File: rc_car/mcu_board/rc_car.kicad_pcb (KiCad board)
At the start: 2 copper layers, 31.1 x 36.2 mm, 22 parts, among them J1 Atmega328, P4 CONN_01X03

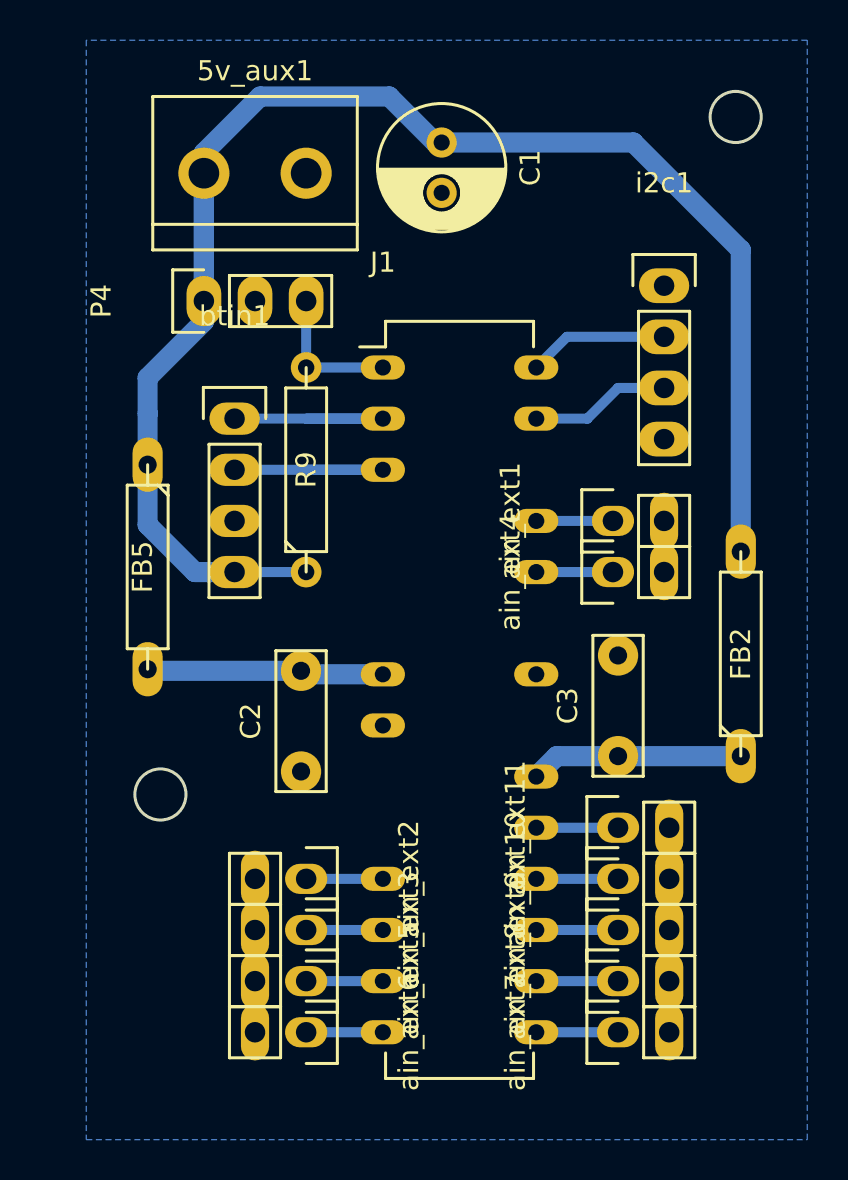
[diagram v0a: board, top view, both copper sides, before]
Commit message: fixes
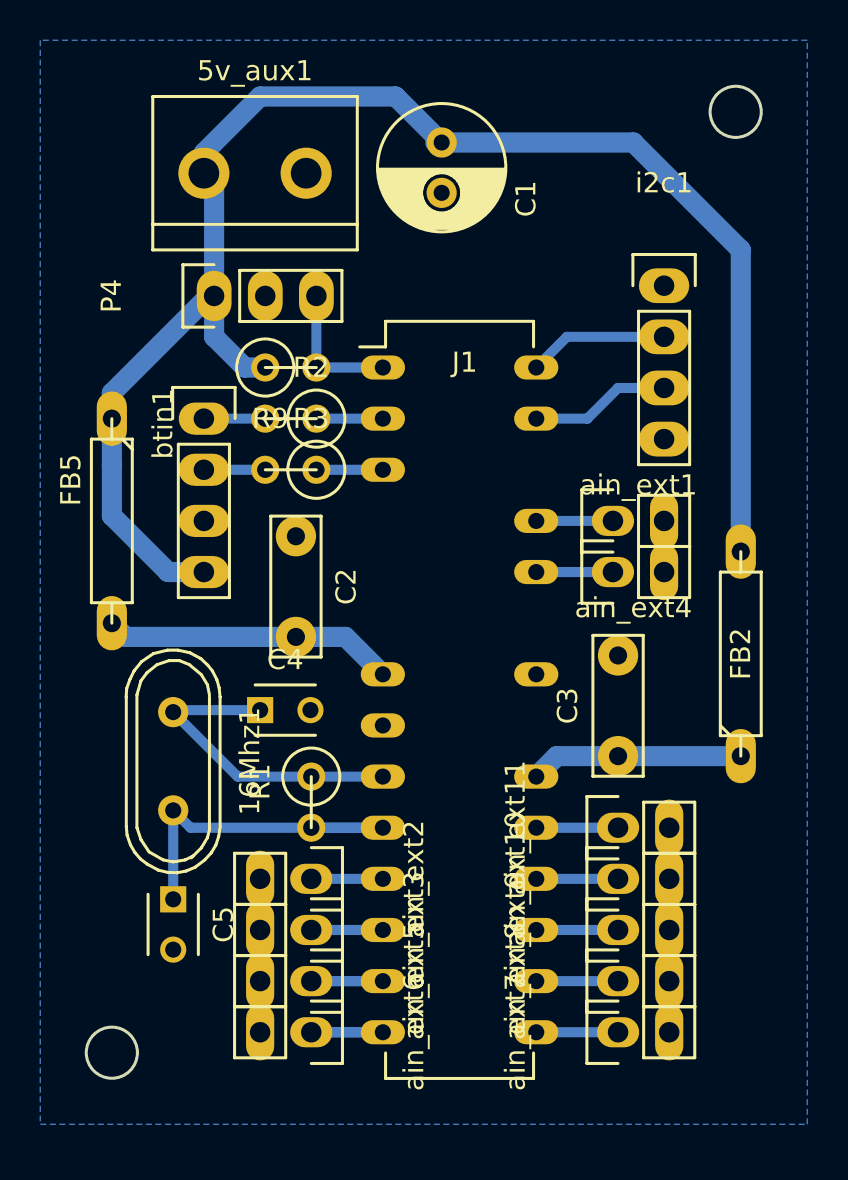
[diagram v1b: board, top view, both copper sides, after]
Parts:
- added 16Mhz1: Crystal_Small, Crystals:Crystal_HC49-U_Vertical, F.Cu at (70.5, 75.8)
- added C4: 22pF, Capacitors_ThroughHole:C_Disc_D3_P2.5, F.Cu at (74.8, 73.3)
- added C5: 22pF, Capacitors_ThroughHole:C_Disc_D3_P2.5, F.Cu at (70.5, 82.7)
- added R1: 1M, Discret:R1, F.Cu at (77.3, 77.9)
- added R2: 1K, Discret:R1, F.Cu at (76.3, 58.8)
- added R3: 1K, Discret:R1, F.Cu at (76.3, 61.3)
- R9: footprint Discret:R4 -> Discret:R1
- moved C2 11.7 mm to (76.6, 64.6), turned to 270 degrees
- moved R9 5.14 mm to (76.3, 56.3), turned to 0 degrees
- moved FB5 2.90 mm to (67.4, 63.9)
- moved btin1 1.52 mm to (72.0, 58.8)
- moved P4 0.57 mm to (72.5, 52.7)
- moved ain_ext2 0.25 mm to (77.3, 81.7)
- moved ain_ext3 0.25 mm to (77.3, 84.2)
- moved ain_ext5 0.25 mm to (77.3, 86.7)
- moved ain_ext6 0.25 mm to (77.3, 89.3)
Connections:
- J1 pad 2: /RX -> Net-(J1-Pad2)
- J1 pad 3: /TX -> Net-(J1-Pad3)
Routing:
- net Net-(16Mhz1-Pad2): track 0.00 -> 18.3 mm
- net Net-(16Mhz1-Pad1): track 0.00 -> 16.1 mm
- net /TX: track 11.2 -> 3.05 mm
- net /RX: track 11.2 -> 3.05 mm
- net /D4: track 3.94 -> 7.49 mm
- net /D3: track 3.81 -> 7.37 mm
- net /D2: track 3.81 -> 7.37 mm
- net Net-(J1-Pad3): track 0.00 -> 3.30 mm
- net Net-(J1-Pad2): track 0.00 -> 3.30 mm
- net /5V: track 83.0 -> 80.5 mm
- net Net-(C2-Pad2): track 12.0 -> 14.5 mm
- net /RST: track 7.58 -> 6.86 mm
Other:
- board size 31.1 x 36.2 mm -> 33.5 x 49.3 mm

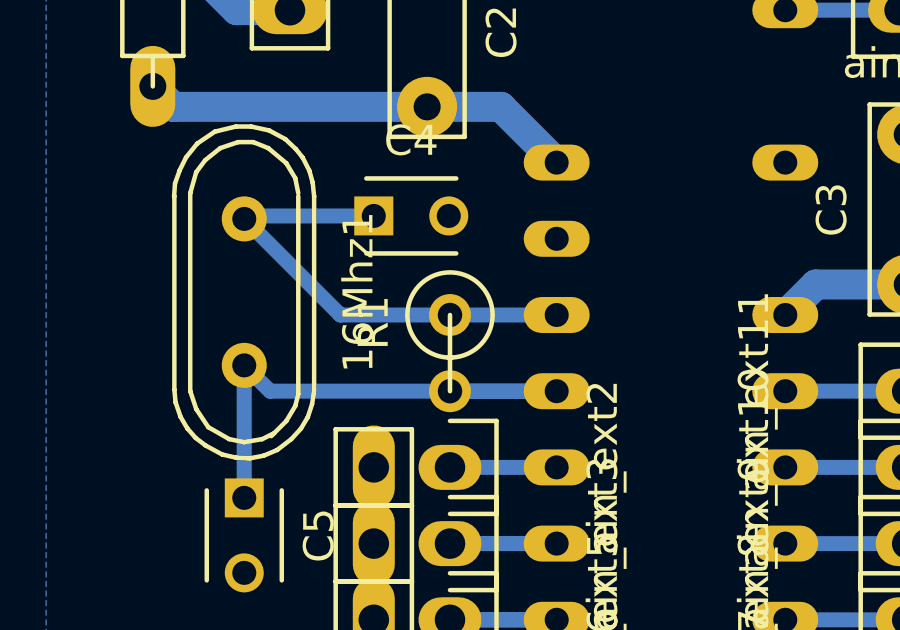
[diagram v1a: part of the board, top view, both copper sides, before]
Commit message: updates
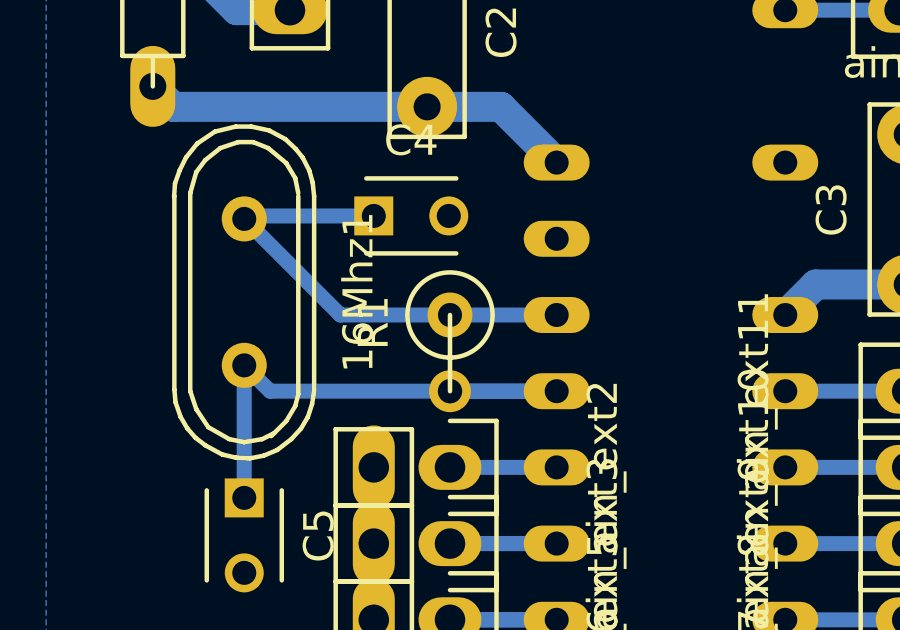
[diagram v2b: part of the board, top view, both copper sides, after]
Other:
- rule pad_to_mask_clearance: 0.2 -> 0
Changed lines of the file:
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@@
-(kicad_pcb (version 4) (host pcbnew 4.0.6)
+(kicad_pcb (version 20171130) (host pcbnew 5.1.4-e60b266~84~ubuntu18.04.1)
   (general
-    (links 57)
-    (no_connects 0)
-    (area 62.36 39.754 101.981001 93.853001)
-    (thickness 1.6)
+    (thickness 1)
     (drawings 2)
     (tracks 68)
@@
     (zone_45_only no)
     (trace_min 0.2)
-    (segment_width 0.2)
-    (edge_width 0.15)
     (via_size 1.2)
     (via_drill 0.8)
@@
     (uvia_min_size 0.2)
     (uvia_min_drill 0.1)
+    (edge_width 0.15)
+    (segment_width 0.2)
     (pcb_text_width 0.3)
     (pcb_text_size 1.5 1.5)
@@
     (mod_text_size 1 1)
     (mod_text_width 0.15)
-    (pad_size 2 2)
-    (pad_drill 0.9)
-    (pad_to_mask_clearance 0.2)
-    (solder_mask_min_width 0.3)
+    (pad_size 1.5 1.5)
+    (pad_drill 0.8)
+    (pad_to_mask_clearance 0)
     (aux_axis_origin 0 0)
     (grid_origin 90.805 164.465)
@@
       (layerselection 0x00030_80000001)
       (usegerberextensions false)
+      (usegerberattributes false)
+      (usegerberadvancedattributes false)
+      (creategerberjobfile false)
       (excludeedgelayer true)
       (linewidth 0.100000)
@@
       (hpglpennumber 1)
       (hpglpenspeed 20)
-      (hpglpendiameter 15)
-      (hpglpenoverlay 2)
+      (hpglpendiameter 15.000000)
       (psnegative false)
       (psa4output false)
@@
       (drillshape 1)
       (scaleselection 1)
-      (outputdirectory output/))
+      (outputdirectory "output/"))
   )
   (net 0 "")
@@
       (effects (font (size 1 1) (thickness 0.15)))
     )
-    (fp_text value 470uF (at -2.794 -2.413 360) (layer F.Fab)
+    (fp_text value 470uF (at -2.794 -2.413) (layer F.Fab)
       (effects (font (size 1 1) (thickness 0.15)))
     )
@@
       (net 1 /5V))
     (model Pin_Headers.3dshapes/Pin_Header_Straight_1x04.wrl
-      (at (xyz 0 -0.15 0))
+      (offset (xyz 0 -3.809999942779541 0))
       (scale (xyz 1 1 1))
       (rotate (xyz 0 0 90))
@@
       (net 2 GND))
     (model Pin_Headers.3dshapes/Pin_Header_Straight_1x02.wrl
-      (at (xyz 0 -0.05 0))
+      (offset (xyz 0 -1.269999980926514 0))
       (scale (xyz 1 1 1))
       (rotate (xyz 0 0 90))
@@
       (net 2 GND))
     (model Pin_Headers.3dshapes/Pin_Header_Straight_1x02.wrl
-      (at (xyz 0 -0.05 0))
+      (offset (xyz 0 -1.269999980926514 0))
       (scale (xyz 1 1 1))
       (rotate (xyz 0 0 90))
@@
       (net 9 /RST))
     (model Pin_Headers.3dshapes/Pin_Header_Straight_1x03.wrl
-      (at (xyz 0 -0.1 0))
+      (offset (xyz 0 -2.539999961853027 0))
       (scale (xyz 1 1 1))
       (rotate (xyz 0 0 90))
@@
       (net 2 GND))
     (model Pin_Headers.3dshapes/Pin_Header_Straight_1x02.wrl
-      (at (xyz 0 -0.05 0))
+      (offset (xyz 0 -1.269999980926514 0))
       (scale (xyz 1 1 1))
       (rotate (xyz 0 0 90))
@@
       (net 2 GND))
     (model Pin_Headers.3dshapes/Pin_Header_Straight_1x02.wrl
-      (at (xyz 0 -0.05 0))
+      (offset (xyz 0 -1.269999980926514 0))
       (scale (xyz 1 1 1))
       (rotate (xyz 0 0 90))
@@
       (net 2 GND))
     (model Pin_Headers.3dshapes/Pin_Header_Straight_1x02.wrl
-      (at (xyz 0 -0.05 0))
+      (offset (xyz 0 -1.269999980926514 0))
       (scale (xyz 1 1 1))
       (rotate (xyz 0 0 90))
@@
       (net 2 GND))
     (model Pin_Headers.3dshapes/Pin_Header_Straight_1x02.wrl
-      (at (xyz 0 -0.05 0))
+      (offset (xyz 0 -1.269999980926514 0))
       (scale (xyz 1 1 1))
       (rotate (xyz 0 0 90))
@@
       (net 2 GND))
     (model Pin_Headers.3dshapes/Pin_Header_Straight_1x02.wrl
-      (at (xyz 0 -0.05 0))
+      (offset (xyz 0 -1.269999980926514 0))
       (scale (xyz 1 1 1))
       (rotate (xyz 0 0 90))
@@
       (net 2 GND))
     (model Pin_Headers.3dshapes/Pin_Header_Straight_1x02.wrl
-      (at (xyz 0 -0.05 0))
+      (offset (xyz 0 -1.269999980926514 0))
       (scale (xyz 1 1 1))
       (rotate (xyz 0 0 90))
@@
       (net 2 GND))
     (model Pin_Headers.3dshapes/Pin_Header_Straight_1x02.wrl
-      (at (xyz 0 -0.05 0))
+      (offset (xyz 0 -1.269999980926514 0))
       (scale (xyz 1 1 1))
       (rotate (xyz 0 0 90))
@@
       (net 2 GND))
     (model Pin_Headers.3dshapes/Pin_Header_Straight_1x02.wrl
-      (at (xyz 0 -0.05 0))
+      (offset (xyz 0 -1.269999980926514 0))
       (scale (xyz 1 1 1))
       (rotate (xyz 0 0 90))
@@
       (net 2 GND))
     (model Pin_Headers.3dshapes/Pin_Header_Straight_1x02.wrl
-      (at (xyz 0 -0.05 0))
+      (offset (xyz 0 -1.269999980926514 0))
       (scale (xyz 1 1 1))
       (rotate (xyz 0 0 90))
@@
       (net 2 GND))
     (model Pin_Headers.3dshapes/Pin_Header_Straight_1x04.wrl
-      (at (xyz 0 -0.15 0))
+      (offset (xyz 0 -3.809999942779541 0))
       (scale (xyz 1 1 1))
       (rotate (xyz 0 0 90))
@@
       (net 2 GND))
     (model Capacitors_ThroughHole.3dshapes/C_Disc_D3_P2.5.wrl
-      (at (xyz 0.0492126 0 0))
+      (offset (xyz 1.250000021226883 0 0))
       (scale (xyz 1 1 1))
       (rotate (xyz 0 0 0))
@@
       (net 2 GND))
     (model Capacitors_ThroughHole.3dshapes/C_Disc_D3_P2.5.wrl
-      (at (xyz 0.0492126 0 0))
+      (offset (xyz 1.250000021226883 0 0))
       (scale (xyz 1 1 1))
       (rotate (xyz 0 0 0))
@@
     (fp_line (start -1.27 0) (end 1.27 0) (layer F.SilkS) (width 0.15))
     (fp_circle (center -1.27 0) (end -0.635 1.27) (layer F.SilkS) (width 0.15))
-    (pad 1 thru_hole circle (at -1.27 0 270) (size 1.397 1.397) (drill 0.8128) (layers *.Cu *.Mask F.SilkS)
+    (pad 1 thru_hole circle (at -1.27 0 270) (size 1.5 1.5) (drill 0.8) (layers *.Cu *.Mask F.SilkS)
       (net 21 "Net-(16Mhz1-Pad1)"))
     (pad 2 thru_hole circle (at 1.27 0 270) (size 1.397 1.397) (drill 0.8128) (layers *.Cu *.Mask F.SilkS)
